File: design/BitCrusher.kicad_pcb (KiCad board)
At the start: 2 copper layers, 181.5 x 86.2 mm, 138 parts, among them J1 BNC, J10 PJ-002BH, J2 BWSMA-KWE-Z001, J3 BWSMA-KE-Z001, J4 BWSMA-KE-Z001, J5 SHOU HAN TYPE-C 14P CC-2.6, J6 Conn_01x04_Pin, J7 Conn_01x04_Pin, J8 Conn_01x03_Pin, J9 Conn_01x03_Pin, Q1 SW4N60, Q2 2SA1213, Q3 GAN080-650EBE, T1 DA2033-AL, U1 STM32F303RETx, U2 USBLC6-2SC6, U3 FT230XQ, U4 TPS7A2050PDQN, U5 TPS7A2033PDQN, U6 LMR33630ADDA, U7 LMR33630ADDA, U8 TLP152TPL_E, U9 MAX22702EASA+

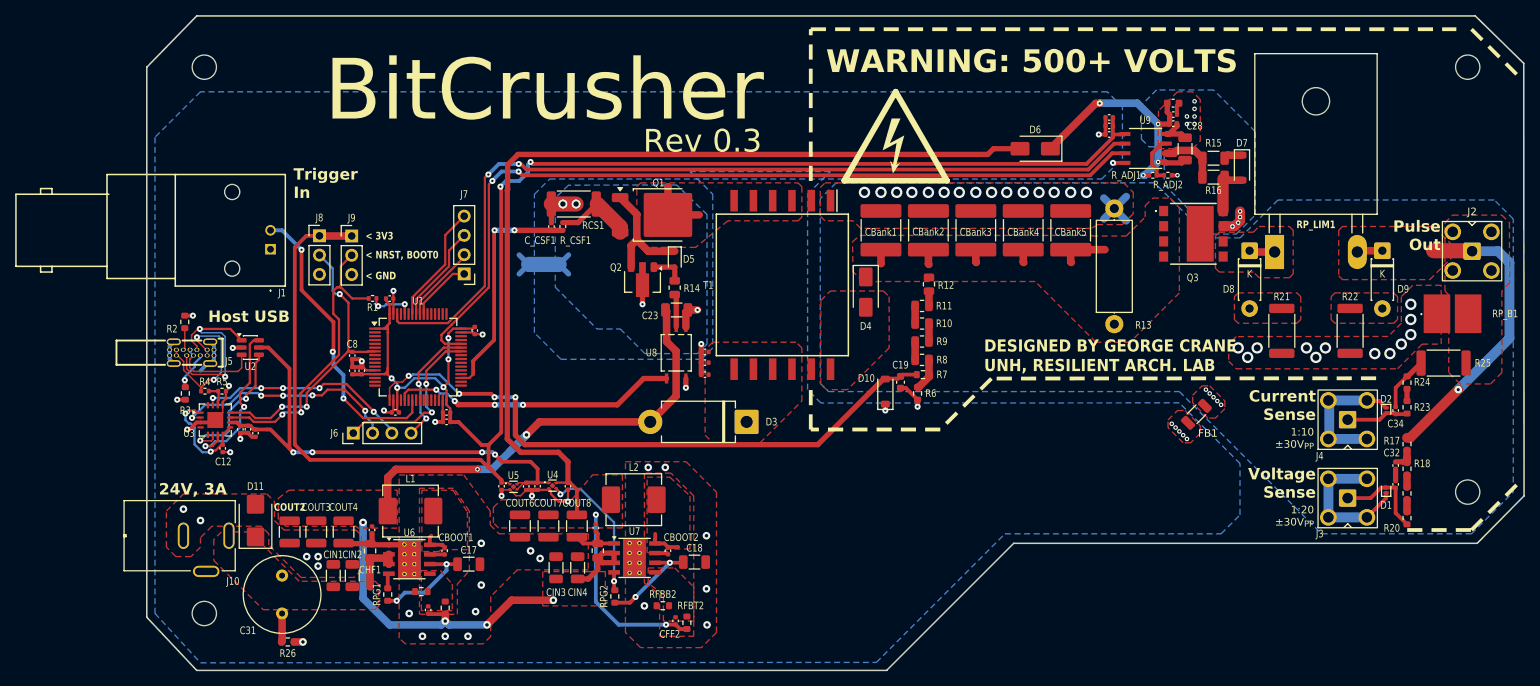
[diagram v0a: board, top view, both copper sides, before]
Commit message: reshaping board
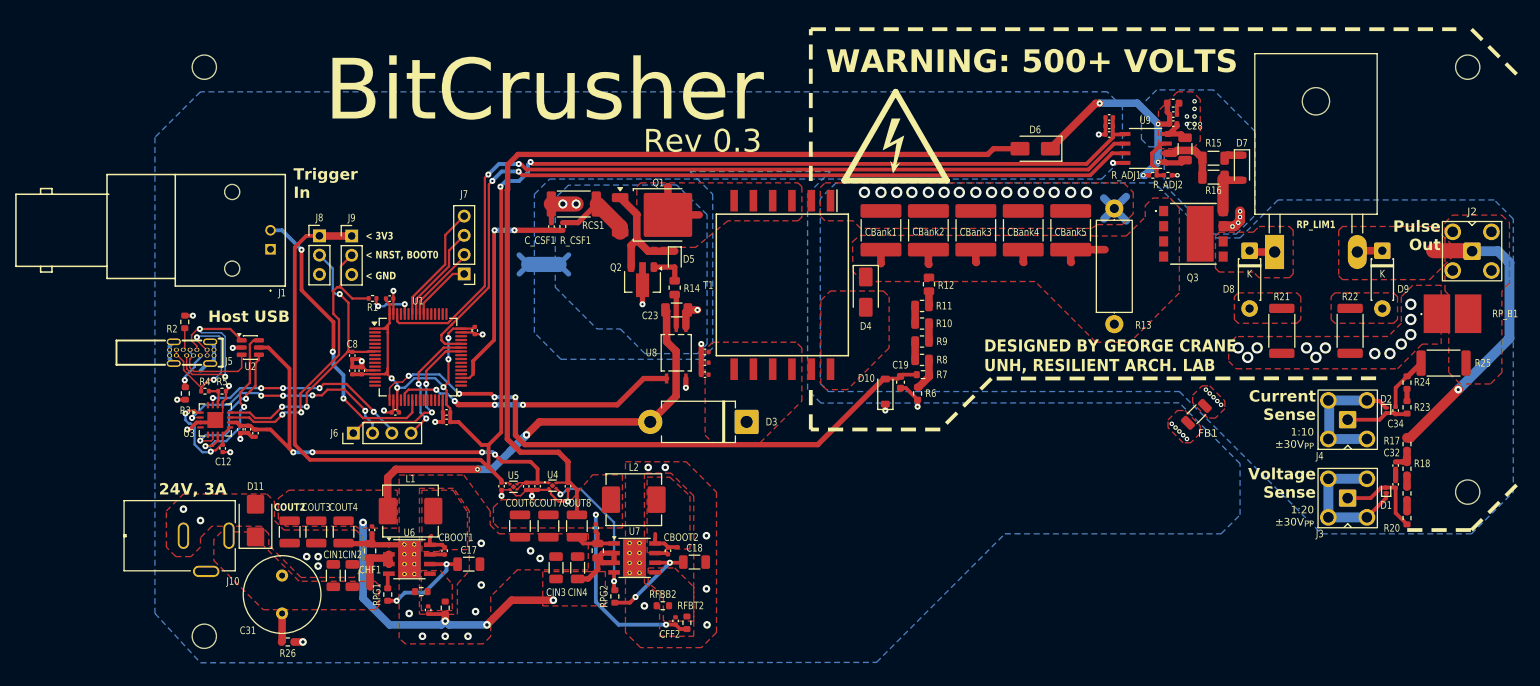
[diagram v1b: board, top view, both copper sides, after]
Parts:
- moved H1 3.00 mm to (66.5, 135.5)
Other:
- board outline removed
